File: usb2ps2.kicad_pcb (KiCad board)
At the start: 2 copper layers, 49 x 44.8 mm, 61 parts, among them CN1 USB, CN2 UART, CN3 PS/2, Q1 BSS138, Q2 BSS138, Q3 BSS138, Q4 BSS138, SW1 Flash Button, SW2 Reset Button, U1 NCP1117-3.3_SOT223, U2 W25Q128JVS, U3 RP2040, Y1 ABM8-272-T3

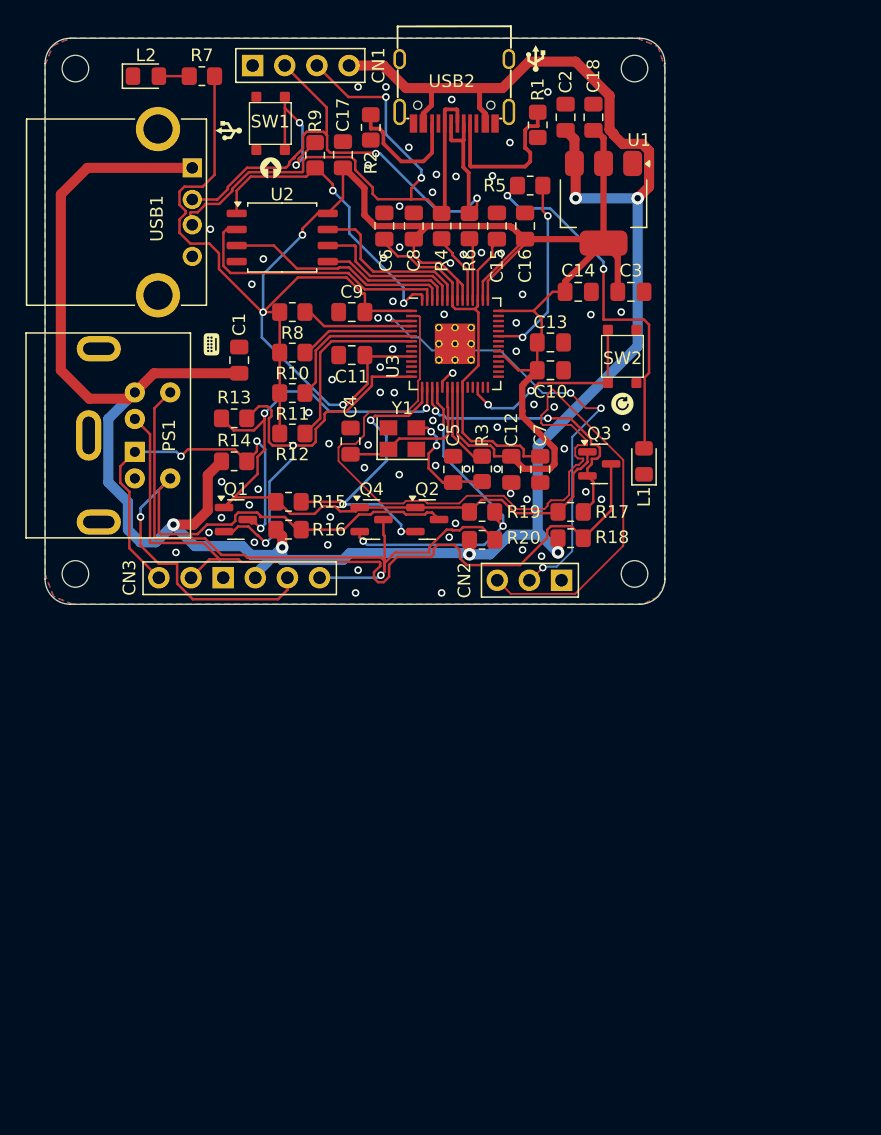
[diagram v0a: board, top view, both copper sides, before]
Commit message: HW Rev 1.2
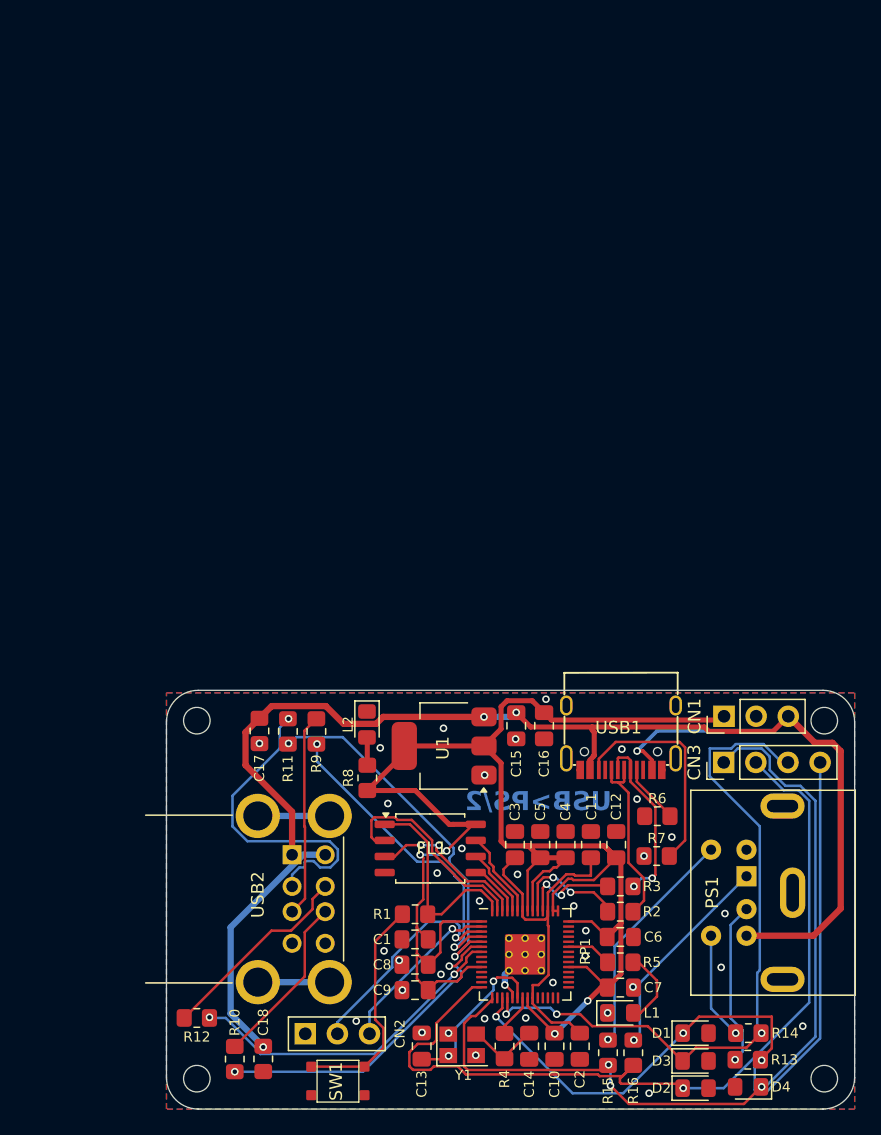
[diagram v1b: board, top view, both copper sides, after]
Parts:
- removed G***: LOGO, LIBS:usb2ps2_logo
- removed Q1, Q2, Q3, Q4: BSS138, Package_TO_SOT_SMD:SOT-23
- removed R17, R18, R19, R20: 10K, Resistor_SMD:R_0805_2012Metric_Pad1.20x1.40mm_HandSolder
- removed REF** (x4): MountingHole_2.1mm, LIBS:MountingHole_2.1mm
- removed SW2: Reset Button, LIBS:Button_SMD_3x3x2
- removed U2: W25Q128JVS, Package_SO:SOIC-8_5.23x5.23mm_P1.27mm
- removed U3: RP2040, LIBS:RP2040-QFN-56
- added D1: 3V3, LIBS:Medved_D_0805, F.Cu at (141.7, 100.4)
- added D2: 3V3, LIBS:Medved_D_0805, F.Cu at (141.7, 104.8)
- added D3: 3V3, LIBS:Medved_D_0805, F.Cu at (141.7, 102.6)
- added D4: 3V3, LIBS:Medved_D_0805, F.Cu at (145.8, 104.7)
- added FL1: W25Q128JVS, LIBS:Medved_SOIC-8_5.23x5.23mm_P1.27mm, F.Cu at (120.7, 85.8)
- added H1: MountingHole, LIBS:MountingHole_2.1mm, F.Cu at (102.2, 75.7)
- added H2: MountingHole, LIBS:MountingHole_2.1mm, F.Cu at (102.2, 104.0)
- added H3: MountingHole, LIBS:MountingHole_2.1mm, F.Cu at (151.8, 104.0)
- added H4: MountingHole, LIBS:MountingHole_2.1mm, F.Cu at (151.8, 75.7)
- added RP1: RP2040, LIBS:RP2040-QFN-56, F.Cu at (128.2, 94.2)
- C1, C2, C3: value 10u -> 100n; footprint Capacitor_SMD:C_0805_2012Metric_Pad1.18x1.45mm_HandSolder -> LIBS:Medved_C_0805
- C10, C6, C7, C8, C9: footprint Capacitor_SMD:C_0805_2012Metric_Pad1.18x1.45mm_HandSolder -> LIBS:Medved_C_0805
- C11, C12: value 100n -> 1u; footprint Capacitor_SMD:C_0805_2012Metric_Pad1.18x1.45mm_HandSolder -> LIBS:Medved_C_0805
- C13, C14: value 100n -> 15p; footprint Capacitor_SMD:C_0805_2012Metric_Pad1.18x1.45mm_HandSolder -> LIBS:Medved_C_0805
- C15, C16: value 1u -> 10u; footprint Capacitor_SMD:C_0805_2012Metric_Pad1.18x1.45mm_HandSolder -> LIBS:Medved_C_0805
- C17: value 100n -> 10u; footprint Capacitor_SMD:C_0805_2012Metric_Pad1.18x1.45mm_HandSolder -> LIBS:Medved_R_0805
- C18: footprint Capacitor_SMD:C_0805_2012Metric_Pad1.18x1.45mm_HandSolder -> LIBS:Medved_R_0805
- C4, C5: value 15p -> 100n; footprint Capacitor_SMD:C_0805_2012Metric_Pad1.18x1.45mm_HandSolder -> LIBS:Medved_C_0805
- CN1: value USB -> Conn_01x03_Pin; footprint LIBS:Medved_USB_Pin4 -> Connector_PinHeader_2.54mm:PinHeader_1x03_P2.54mm_Vertical
- CN3: value PS/2 -> PS/2 Pins; footprint LIBS:Medved_PS2_Con6 -> Connector_PinHeader_2.54mm:PinHeader_1x04_P2.54mm_Vertical
- L1, L2: footprint LED_SMD:LED_0805_2012Metric_Pad1.15x1.40mm_HandSolder -> LIBS:Medved_LED_0805
- R1: value 5.1K -> 1k; footprint Resistor_SMD:R_0805_2012Metric_Pad1.20x1.40mm_HandSolder -> LIBS:Medved_R_0805
- R10, R11, R12: value 10K -> 22R; footprint Resistor_SMD:R_0805_2012Metric_Pad1.20x1.40mm_HandSolder -> LIBS:Medved_R_0805
- R13, R14, R15, R16: value 10K -> 100R; footprint Resistor_SMD:R_0805_2012Metric_Pad1.20x1.40mm_HandSolder -> LIBS:Medved_R_0805
- R2: value 5.1K -> 27; footprint Resistor_SMD:R_0805_2012Metric_Pad1.20x1.40mm_HandSolder -> LIBS:Medved_R_0805
- R3: value 1k -> 27; footprint Resistor_SMD:R_0805_2012Metric_Pad1.20x1.40mm_HandSolder -> LIBS:Medved_R_0805
- R4: value 27 -> 1k; footprint Resistor_SMD:R_0805_2012Metric_Pad1.20x1.40mm_HandSolder -> LIBS:Medved_R_0805
- R5: footprint Resistor_SMD:R_0805_2012Metric_Pad1.20x1.40mm_HandSolder -> LIBS:Medved_R_0805
- R6: value 27 -> 5.1K; footprint Resistor_SMD:R_0805_2012Metric_Pad1.20x1.40mm_HandSolder -> LIBS:Medved_R_0805
- R7: value 1K -> 5.1K; footprint Resistor_SMD:R_0805_2012Metric_Pad1.20x1.40mm_HandSolder -> LIBS:Medved_R_0805
- R8: value 10K -> 1K; footprint Resistor_SMD:R_0805_2012Metric_Pad1.20x1.40mm_HandSolder -> LIBS:Medved_R_0805
- R9: value 1k -> 22R; footprint Resistor_SMD:R_0805_2012Metric_Pad1.20x1.40mm_HandSolder -> LIBS:Medved_R_0805
- U1: footprint Package_TO_SOT_SMD:SOT-223-3_TabPin2 -> LIBS:Medved_SOT-223-3_TabPin2
- USB1: value USB_A -> USB Type C; footprint Connector_USB:USB_A_CONNFLY_DS1095-WNR0 -> LIBS:USB-TYPE-C-31-M-12_lib2
- USB2: value USB Type C -> USB_A_Stacked; footprint LIBS:USB-TYPE-C-31-M-12_lib2 -> LIBS:Medved_USB_A_CUI_UJ2-ADH-TH_Horizontal_Stacked
- moved C18 78.9 mm to (107.5, 102.4), turned to -90 degrees
- moved SW1 76.2 mm to (115.1, 105.8), turned to 180 degrees
- moved C2 73.4 mm to (132.5, 101.4), turned to -90 degrees
- moved R7 71.4 mm to (138.6, 86.4)
- moved USB2 66.7 mm to (109.8, 86.3), turned to 0 degrees
- moved R2 65.1 mm to (135.7, 90.8), turned to 180 degrees
- moved R4 65.0 mm to (126.6, 101.4)
- moved R13 65.0 mm to (145.8, 102.5)
- moved R1 63.1 mm to (119.5, 91.0), turned to 180 degrees
- moved R5 61.8 mm to (135.7, 94.8), turned to 180 degrees
- moved R14 60.8 mm to (145.8, 100.4)
- moved C14 59.8 mm to (128.5, 101.4), turned to -90 degrees
- moved CN1 59.4 mm to (143.9, 75.3), turned to 90 degrees
- moved C6 59.2 mm to (135.7, 92.8), turned to 0 degrees
- moved PS1 58.9 mm to (145.7, 88.0), turned to 90 degrees
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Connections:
- C1 pad 1: VBUS -> +3V3
- C11 pad 1: +3V3 -> Net-(RP1-VREG_VOUT)
- C13 pad 1: +3V3 -> /RP2040/XIN
- C14 pad 1: +3V3 -> Net-(C14-Pad1)
- C15 pad 1: +1V1 -> VBUS
- C17 pad 1: +3V3 -> VBUS
- C18 pad 1: +3V3 -> VBUS
- C2 pad 1: VBUS -> Net-(RP1-VREG_VOUT)
- C3 pad 1: +3V3 -> Net-(RP1-VREG_VOUT)
- C4 pad 1: /XIN -> +3V3
- C5 pad 1: Net-(C5-Pad1) -> +3V3
- C6 pad 1: +1V1 -> +3V3
- C7 pad 1: +1V1 -> +3V3
- CN1 pad 1: VBUS -> +3V3
- CN1 pad 2: /D+ -> GND
- CN1 pad 3: /D- -> VBUS
- CN3 pad 1: /KB_DATA -> /GPIO12
- CN3 pad 2: /MS_DATA -> /GPIO11
- CN3 pad 3: GND -> /GPIO15
- CN3 pad 4: VBUS -> /GPIO14
- PS1 pad 1: /KB_DATA -> /PS2 with Diodes/KB_DATA
- PS1 pad 2: /MS_DATA -> /PS2 with Diodes/MS_DATA
- PS1 pad 5: /KB_CLK -> /PS2 with Diodes/KB_CLK
- PS1 pad 6: /MS_CLK -> /PS2 with Diodes/MS_CLK
- R1 pad 1: GND -> /RP2040/QSPI_SS
- R1 pad 2: Net-(USB2-CC1) -> /RP2040/~{USB_BOOT}
- R10 pad 1: /GPIO3 -> /GPIO4
- R10 pad 2: +3V3 -> Net-(USB2-D2+)
- R11 pad 1: /GPIO4 -> /GPIO3
- R11 pad 2: +3V3 -> Net-(USB2-D1-)
- R12 pad 2: +3V3 -> Net-(USB2-D2-)
- R13 pad 1: /GPIO13 -> /PS2 with Diodes/MS_DATA
- R13 pad 2: /GPIO11 -> /GPIO14
- R14 pad 1: VBUS -> /PS2 with Diodes/MS_CLK
- R14 pad 2: /KB_DATA -> /GPIO15
- R15 pad 1: /GPIO13 -> /PS2 with Diodes/KB_CLK
- R16 pad 1: VBUS -> /PS2 with Diodes/KB_DATA
- R16 pad 2: /KB_CLK -> /GPIO11
- R2 pad 1: GND -> /D+
- R2 pad 2: Net-(USB2-CC2) -> Net-(RP1-USB_DP)
- R3 pad 1: /XOUT -> /D-
- R3 pad 2: Net-(C5-Pad1) -> Net-(RP1-USB_DM)
- R4 pad 1: /D+ -> /RP2040/XOUT
- R4 pad 2: Net-(U3-USB_DP) -> Net-(C14-Pad1)
- R5 pad 2: /GPIO25 -> /RP2040/GPIO25
- R6 pad 1: /D- -> GND
- R6 pad 2: Net-(U3-USB_DM) -> Net-(USB1-CC1)
- R7 pad 1: Net-(L2-A) -> GND
- R7 pad 2: +3V3 -> Net-(USB1-CC2)
- R8 pad 1: /GPIO2 -> Net-(L2-A)
- R9 pad 1: /QSPI_SS -> /GPIO2
- R9 pad 2: /~{USB_BOOT} -> Net-(USB2-D1+)
- SW1 pad 2: /~{USB_BOOT} -> GND
- SW1 pad 3: GND -> /RP2040/~{USB_BOOT}
- SW1 pad 4: /~{USB_BOOT} -> /RP2040/~{USB_BOOT}
- USB1 pad 1: VBUS -> GND
- USB1 pad 2: /D- -> VBUS
- USB1 pad 3: /D+ -> unconnected-(USB1-SBU2-Pad3)
- USB1 pad 4: GND -> Net-(USB1-CC1)
- USB1 pad 5: GND -> /D-
- USB2 pad 1: GND -> VBUS
- USB2 pad 2: VBUS -> Net-(USB2-D1-)
- USB2 pad 3: unconnected-(USB2-SBU2-Pad3) -> Net-(USB2-D1+)
- USB2 pad 4: Net-(USB2-CC1) -> GND
- USB2 pad 5: /D- -> VBUS
- USB2 pad 6: /D+ -> Net-(USB2-D2-)
- USB2 pad 7: /D- -> Net-(USB2-D2+)
- USB2 pad 8: /D+ -> GND
- USB2 pad 9: unconnected-(USB2-SBU1-Pad9) -> GND
- Y1 pad 1: /XIN -> /RP2040/XIN
- Y1 pad 3: Net-(C5-Pad1) -> Net-(C14-Pad1)
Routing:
- net VBUS: track 192.4 -> 122.6 mm, vias 6 -> 4
- net /GPIO0: track 78.2 -> 13.5 mm, vias 0 -> 1
- net /GPIO13: track 64.1 -> 0.00 mm, vias 2 -> 0
- net /MS_DATA: track 61.9 -> 0.00 mm
- net /MS_CLK: track 52.5 -> 0.00 mm, vias 1 -> 0
- net /KB_CLK: track 51.2 -> 0.00 mm, vias 1 -> 0
- net +3V3: track 187.1 -> 143.0 mm, vias 3 -> 4
- net /GPIO12: track 24.7 -> 67.1 mm
- net /GPIO14: track 22.7 -> 63.8 mm, vias 2 -> 3
- net /D+: track 52.4 -> 14.3 mm, vias 2 -> 0
- net /GPIO11: track 32.7 -> 69.5 mm, vias 2 -> 1
- net +1V1: track 34.6 -> 0.00 mm
- net /D-: track 47.0 -> 14.1 mm
- net /KB_DATA: track 31.9 -> 0.00 mm, vias 3 -> 0
- net /GPIO15: track 27.3 -> 55.9 mm
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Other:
- board size 49 x 44.8 mm -> 54.4 x 33.1 mm
- board text added: "HW Rev 1.2"
- board text added: "USB>PS/2"
- board text added: "rh1.dev"
- board text removed: "HW Rev 1.1"
- board text removed: "© 2024 Mikhail Matveev https://rh1.dev"
